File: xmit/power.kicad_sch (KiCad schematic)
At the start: 27 parts, among them Q301 GSF3407, U202 74LVC1G66, U203 74LVC1G66, U204 74LVC1G66, U205 74LVC1G66, U206 74LVC1G66, U207 74LVC1G66, U208 74LVC1G66, U209 74LVC1G66, U301 TLV760, U302 L7812, U303 TPS7A20xxxDBV

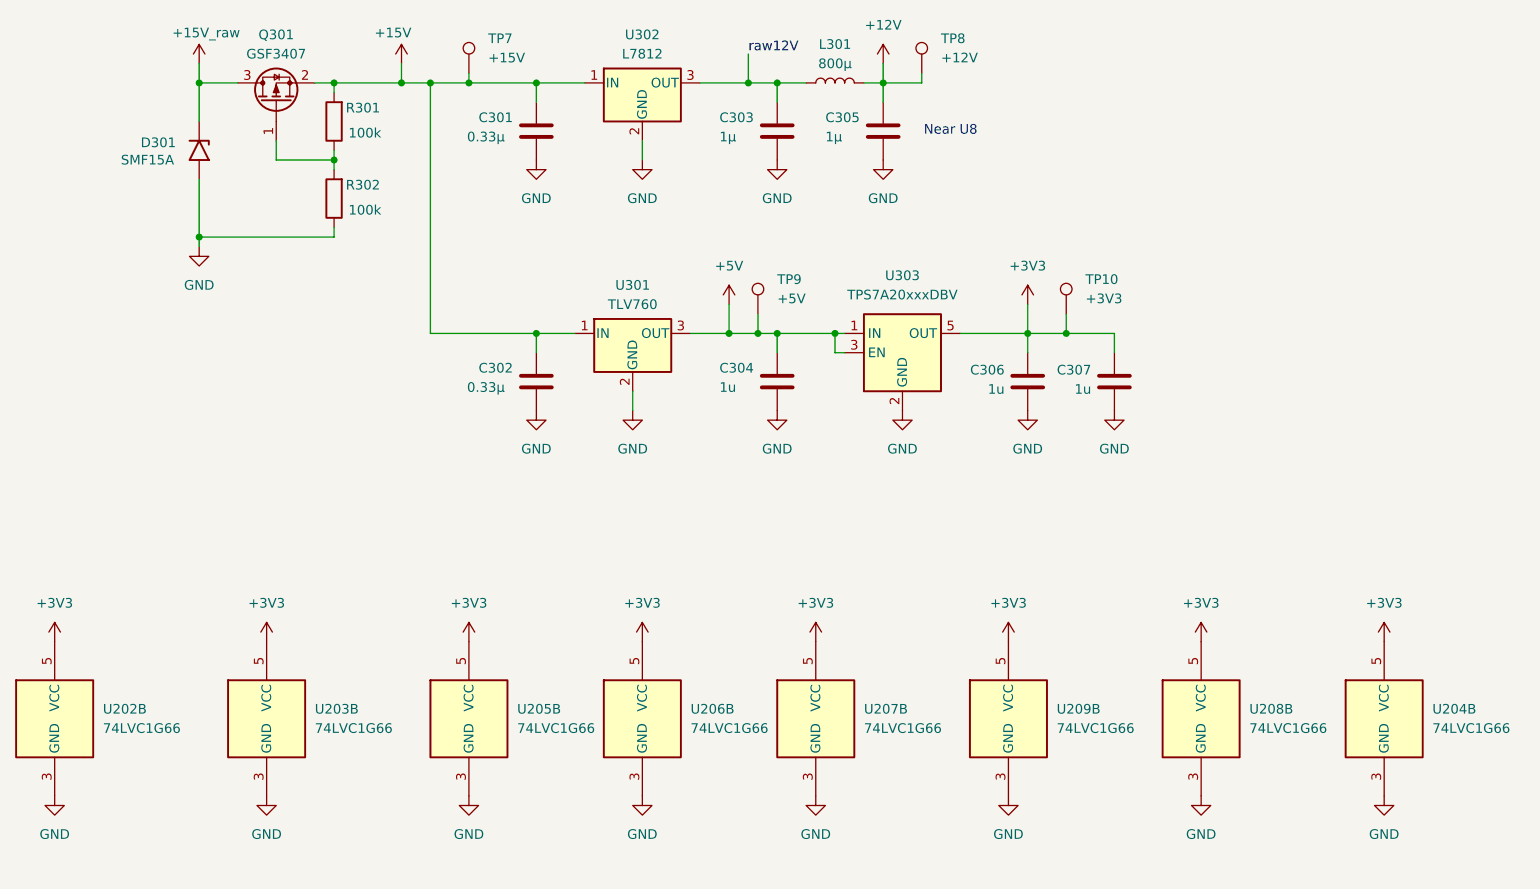
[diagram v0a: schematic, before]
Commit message: changes up to first spin
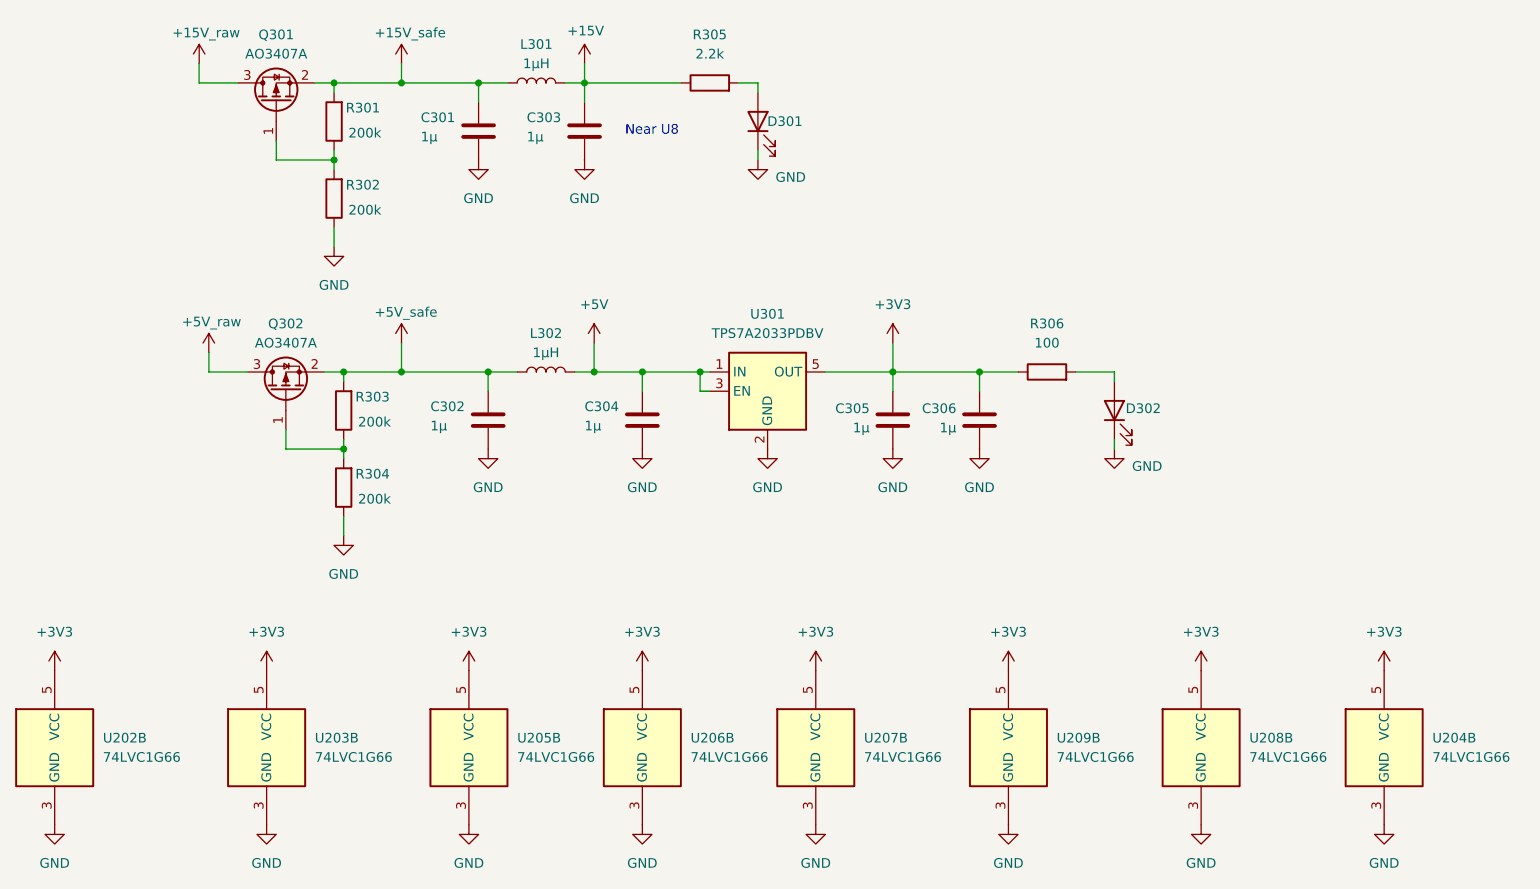
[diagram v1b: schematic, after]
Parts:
- removed C301: 0.33µ, Capacitor_SMD:C_0805_2012Metric, symbol Device:C
- removed D301: SMF15A, Diode_SMD:D_SMF, symbol Diode:SMF5V0A
- removed TP10: +3V3, TestPoint:TestPoint_Pad_1.0x1.0mm, symbol Connector:TestPoint
- removed TP7: +15V, TestPoint:TestPoint_Pad_1.0x1.0mm, symbol Connector:TestPoint
- removed TP8: +12V, TestPoint:TestPoint_Pad_1.0x1.0mm, symbol Connector:TestPoint
- removed TP9: +5V, TestPoint:TestPoint_Pad_1.0x1.0mm, symbol Connector:TestPoint
- removed U301: TLV760, Package_TO_SOT_SMD:TSOT-23, symbol Regulator_Linear:L7805
- removed U302: L7812, Package_TO_SOT_THT:TO-220-3_Horizontal_TabDown, symbol Regulator_Linear:L7812
- added D301, D302: LED, LED_SMD:LED_0603_1608Metric, symbol Device:LED
- added L302: 1µH, Inductor_SMD:L_0805_2012Metric_Pad1.05x1.20mm_HandSolder, symbol Device:L
- added Q302: AO3407A, Package_TO_SOT_SMD:SOT-23, symbol Transistor_FET:DMP3099L
- added R303, R304: 200k, Resistor_SMD:R_0805_2012Metric_Pad1.20x1.40mm_HandSolder, symbol Device:R
- added R305: 2.2k, Resistor_SMD:R_0603_1608Metric, symbol Device:R
- added R306: 100, Resistor_SMD:R_0603_1608Metric, symbol Device:R
- C301: renamed from C303; KiLib_Generator (none) -> SMD_2terminal_chip_molded; LCSC Part # (none) -> C76645; now left out of the parts list
- C302: value 0.33µ -> 1µ; KiLib_Generator (none) -> SMD_2terminal_chip_molded; LCSC Part # (none) -> C76645; now left out of the parts list
- C303: renamed from C305; KiLib_Generator (none) -> SMD_2terminal_chip_molded; LCSC Part # (none) -> C76645; now left out of the parts list
- C304: value 1u -> 1µ; KiLib_Generator (none) -> SMD_2terminal_chip_molded; LCSC Part # (none) -> C76645; now left out of the parts list
- C305: renamed from C306; value 1u -> 1µ; KiLib_Generator (none) -> SMD_2terminal_chip_molded; LCSC Part # (none) -> C76645; now left out of the parts list
- C306: renamed from C307; value 1u -> 1µ; KiLib_Generator (none) -> SMD_2terminal_chip_molded; LCSC Part # (none) -> C76645; now left out of the parts list
- L301: value 800µ -> 1µH; KiLib_Generator (none) -> SMD_2terminal_chip_molded; LCSC Part # (none) -> C19533; now left out of the parts list
- Q301: value GSF3407 -> AO3407A; KiLib_Generator (none) -> package/gullwing; LCSC Part # (none) -> C15155; now left out of the parts list
- R301, R302: value 100k -> 200k; KiLib_Generator (none) -> SMD_2terminal_chip_molded; LCSC Part # (none) -> C17539; now left out of the parts list
- U202, U203, U204, U205, U206, U207, U208, U209: footprint Package_TO_SOT_SMD:SOT-23-5_HandSoldering -> Package_TO_SOT_SMD:SOT-23-5; KiLib_Generator (none) -> package/gullwing; LCSC Part # (none) -> C113518
- U301: renamed from U303; value TPS7A20xxxDBV -> TPS7A2033PDBV; KiLib_Generator (none) -> package/gullwing; LCSC Part # (none) -> C7827; now left out of the parts list
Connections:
- net +12V is gone; now on net +15V: C303.2, L301.2
- net +15V: now also R305.1; no longer C302.2, Q301.2 (S), R301.2
- net +3V3: now also R306.1
- net +5V: now also L302.2
- net GND: now also D301.1 (K), D302.1 (K), R304.1
- net raw12V renamed +15V_safe
- net +15V_safe: now also Q301.2 (S), R301.2
- new net: Q302.1 (G), R303.1, R304.2
- new net: D301.2 (A), R305.2
- new net: D302.2 (A), R306.2
- new net +5V_raw: Q302.3 (D)
- new net +5V_safe: C302.2, L302.1, Q302.2 (S), R303.2
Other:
- moved on the sheet: C301, C303, C304, C305, C306, L301, U202B, U203B, U204B, U205B, U206B, U207B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
